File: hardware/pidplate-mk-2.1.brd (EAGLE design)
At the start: 50 x 50 mm, 35 parts, among them Q1 2N7000, U1 ATMEGA328P, U2 MAX31855, U3 VSK-S1-3.3V

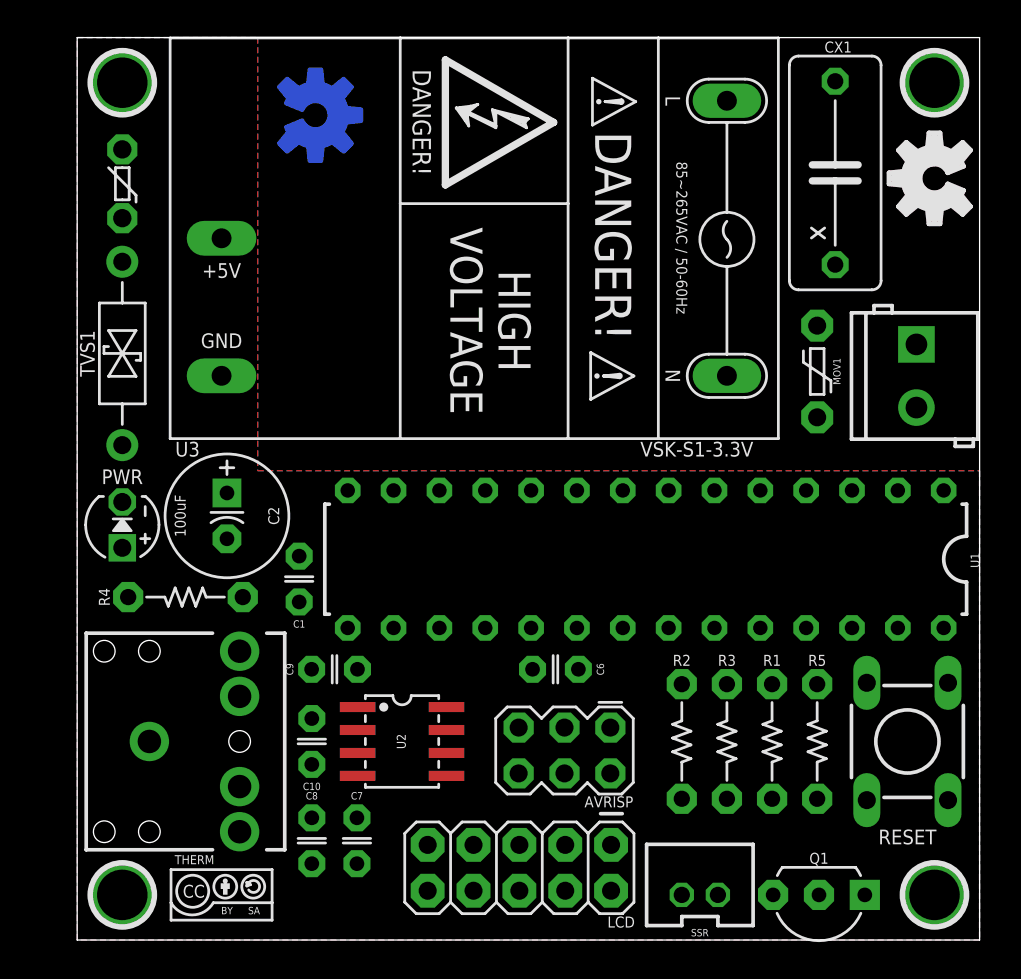
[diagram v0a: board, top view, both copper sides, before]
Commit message: mini mini mini
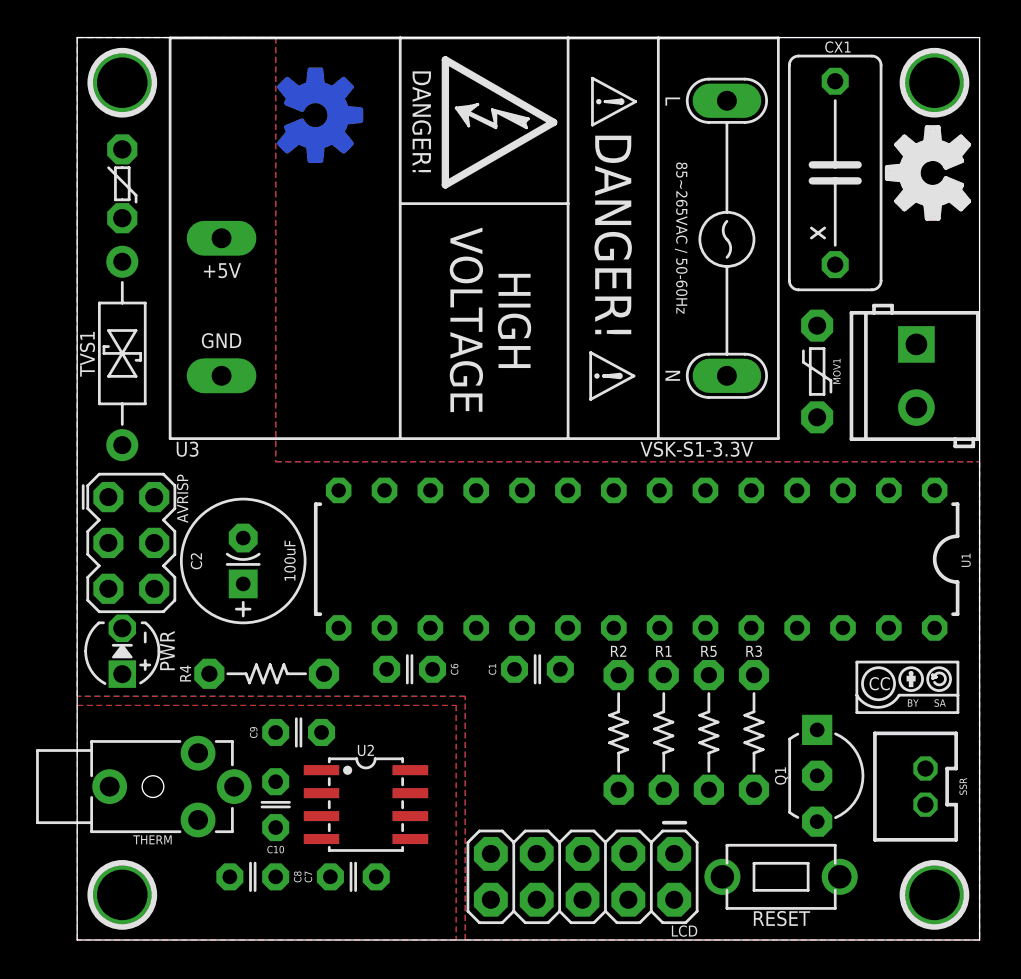
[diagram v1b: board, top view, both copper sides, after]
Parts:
- RESET: value SPST-NO-TACT6MM-PTH -> SPST-NO-TACT3MM-PTH-SMALL-PADS; device A_butts:DTS-6 -> A_butts:DTS-3-SMALL-PADS
- THERM: device A_butts:AUDIO-JACK -> A_butts:STEREOJACK2.5MM_STEREOJACK2.5MM
- moved U$2 39.7 mm to (46.0, 14.0)
- moved AVRISP 26.6 mm to (3.00, 22.0), turned to 270 degrees
- moved C1 14.1 mm to (25.5, 15.0), turned to 0 degrees
- moved SSR 13.9 mm to (47.0, 8.50), turned to 90 degrees
- moved RESET 10.3 mm to (39.0, 3.50), turned to 180 degrees
- moved C6 8.08 mm to (18.4, 15.0)
- moved PWR 7.00 mm to (2.50, 16.0)
- moved Q1 6.60 mm to (41.0, 9.10), turned to 270 degrees
- moved R4 6.19 mm to (10.5, 14.8)
- moved R1 6.02 mm to (32.5, 11.5)
- moved R5 6.02 mm to (35.0, 11.5)
- moved C10 4.03 mm to (11.0, 7.50)
- moved U2 4.03 mm to (16.0, 7.50)
- moved C9 4.03 mm to (12.3, 11.5)
- moved C8 3.83 mm to (9.73, 3.50), turned to 180 degrees
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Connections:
- net 3.3V: now also R1.P$1; no longer R1.P$2
- net GND: now also R5.P$2, THERM.SHIELD; no longer R5.P$1, RESET.2, THERM.SLEEVE
- net N$6: now also SSR.2; no longer SSR.1
- net N$9: now also SSR.1; no longer SSR.2
- net RESET: now also R1.P$2, RESET.2; no longer R1.P$1, RESET.3, RESET.4
- net SSR: now also R5.P$1; no longer R5.P$2
- net TC+/YELLOW: now also THERM.RING1, THERM.RING2; no longer THERM.TIP
- net TC-/RED: now also THERM.TIP; no longer THERM.RING
